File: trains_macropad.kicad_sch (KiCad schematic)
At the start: 17 parts, among them SW1 SW_Push, SW2 SW_Push, SW3 SW_Push, SW4 SW_Push, SW5 RotaryEncoder_Switch, SW6 RotaryEncoder_Switch, U1 MCU_Seeed_XIAO_RP2040, U2 MCP23017_SP

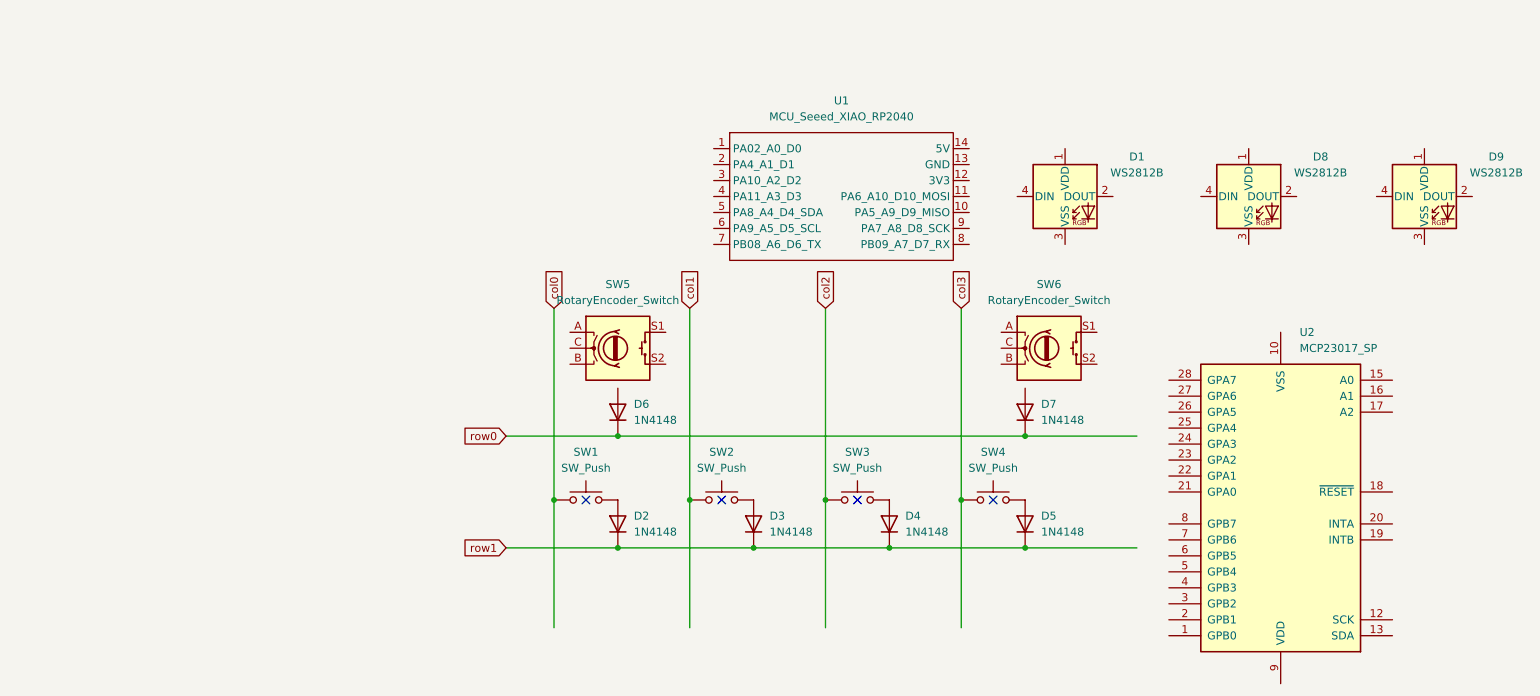
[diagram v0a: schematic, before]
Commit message: I DID IT
ALL THE THINGS EXCEPT CAD AND FIRMWARE....except cad and firmware.............i am going to go cry
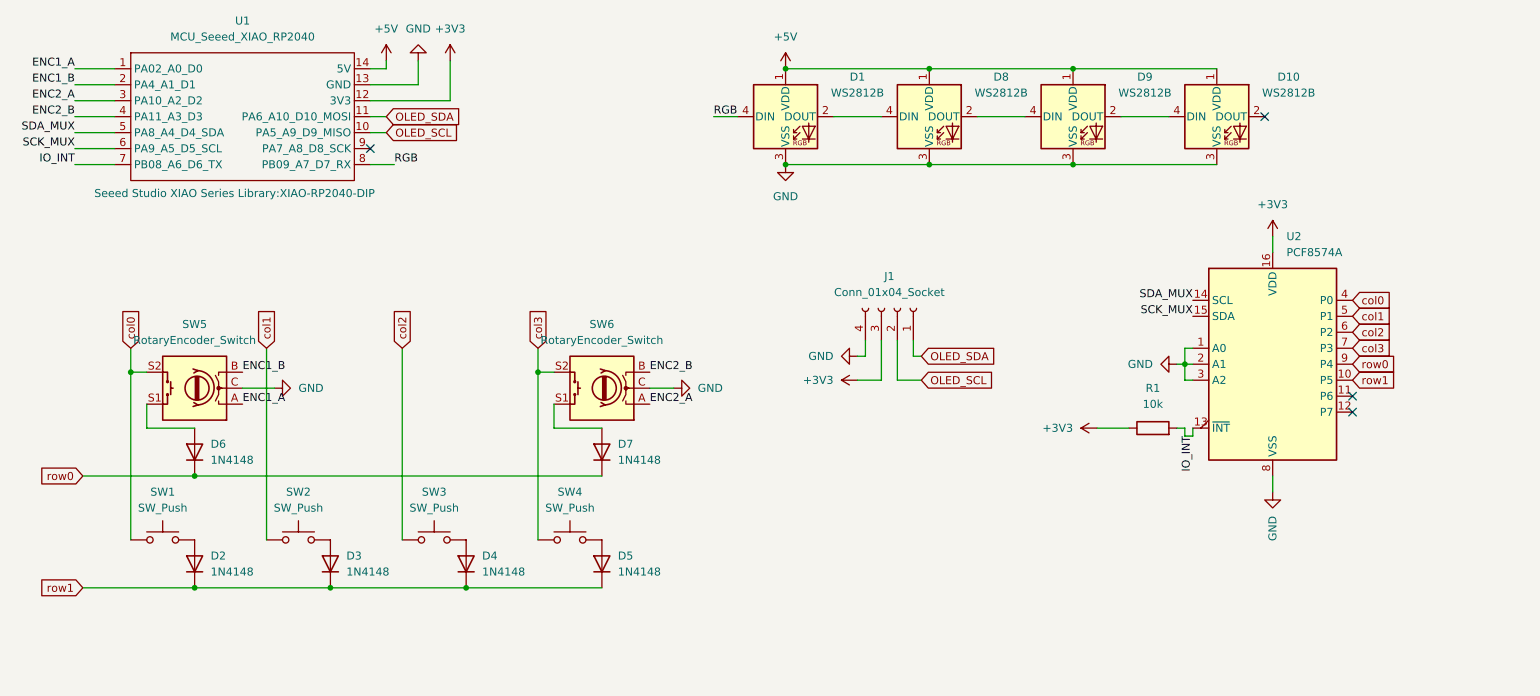
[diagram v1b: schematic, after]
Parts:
- removed U2: MCP23017_SP, Package_DIP:DIP-28_W7.62mm, symbol Interface_Expansion:MCP23017_SP
- added D10: WS2812B, Keebio-Parts:SK6812-MINI-E, symbol LED:WS2812B
- added J1: Conn_01x04_Socket, Connector_PinSocket_2.54mm:PinSocket_1x04_P2.54mm_Vertical, symbol Connector:Conn_01x04_Socket
- added R1: 10k, Resistor_THT:R_Axial_DIN0207_L6.3mm_D2.5mm_P10.16mm_Horizontal, symbol Device:R
- added U2: PCF8574A, Package_DIP:DIP-16_W7.62mm, symbol Interface_Expansion:PCF8574A
- D1, D8, D9: footprint LED_SMD:LED_WS2812B_PLCC4_5.0x5.0mm_P3.2mm -> Keebio-Parts:SK6812-MINI-E
- SW1, SW2, SW3, SW4: footprint (none) -> MX_Only:MXOnly-1U-Hotswap-Antishear
- SW5, SW6: footprint (none) -> Keebio-Parts:RotaryEncoder_EC11
- U1: footprint (none) -> Seeed Studio XIAO Series Library:XIAO-RP2040-DIP
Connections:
- net col0: now also SW5.S2, U2.4 (P0)
- net col1: now also U2.5 (P1)
- net col2: now also U2.6 (P2)
- net col3: now also SW6.S2, U2.7 (P3)
- net row0: now also U2.9 (P4)
- net row1: now also U2.10 (P5)
- net ENC1_A: now reaches U1.1 (PA02_A0_D0)
- net ENC1_A: now also SW5.A
- net OLED_SCL: now reaches U1.10 (PA5_A9_D9_MISO)
- net OLED_SCL: now also J1.2 (Pin_2)
- net OLED_SDA: now reaches U1.11 (PA6_A10_D10_MOSI)
- net OLED_SDA: now also J1.1 (Pin_1)
- net +3V3: now reaches U1.12 (3V3)
- net +3V3: now also J1.3 (Pin_3), R1.1, U2.16 (VDD)
- net GND: now reaches U1.13 (GND)
- net GND: now also D1.3 (VSS), D8.3 (VSS), D9.3 (VSS), SW5.C, SW6.C, D10.3 (VSS), J1.4 (Pin_4), U2.1 (A0), U2.2 (A1), U2.3 (A2), U2.8 (VSS)
- net +5V: now reaches U1.14 (5V)
- net +5V: now also D1.1 (VDD), D8.1 (VDD), D9.1 (VDD), D10.1 (VDD)
- net ENC1_B: now reaches U1.2 (PA4_A1_D1)
- net ENC1_B: now also SW5.B
- net ENC2_A: now reaches U1.3 (PA10_A2_D2)
- net ENC2_A: now also SW6.A
- net ENC2_B: now reaches U1.4 (PA11_A3_D3)
- net ENC2_B: now also SW6.B
- net SDA_MUX: now reaches U1.5 (PA8_A4_D4_SDA)
- net SDA_MUX: now also U2.14 (SCL)
- net SCK_MUX: now reaches U1.6 (PA9_A5_D5_SCL)
- net SCK_MUX: now also U2.15 (SDA)
- net IO_INT: now reaches U1.7 (PB08_A6_D6_TX)
- net IO_INT: now also R1.2, U2.13 (~{INT})
- net RGB: now reaches U1.8 (PB09_A7_D7_RX)
- net RGB: now also D1.4 (DIN)
- net at D9.2 (DOUT): now also D10.4 (DIN)
- net at D9.4 (DIN): now also D8.2 (DOUT)
- net at SW6.S1: now also D7.2 (A)
- net at SW5.S1: now also D6.2 (A)
- net at D8.4 (DIN): now also D1.2 (DOUT)
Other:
- moved on the sheet: D1, D2, D3, D4, D5, D6, D7, D8, D9, SW1, SW2, SW3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
